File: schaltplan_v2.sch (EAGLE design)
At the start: 43 parts, among them T1 2N3565, T2 2N3565, T3 2N3565, T4 2N3565, T5 2N3565, T6 2N3565, T7 2N3565, T8 2N3565, X1 SSW-102-02-S-S-RA, X2 SSW-102-02-S-S-RA, X3 SSW-103-02-S-S-RA, X4 SSW-109-02-S-S-RA, X5 SSW-103-02-S-S-RA, X6 SSW-103-02-S-S-RA, X7 SSW-103-02-S-S-RA

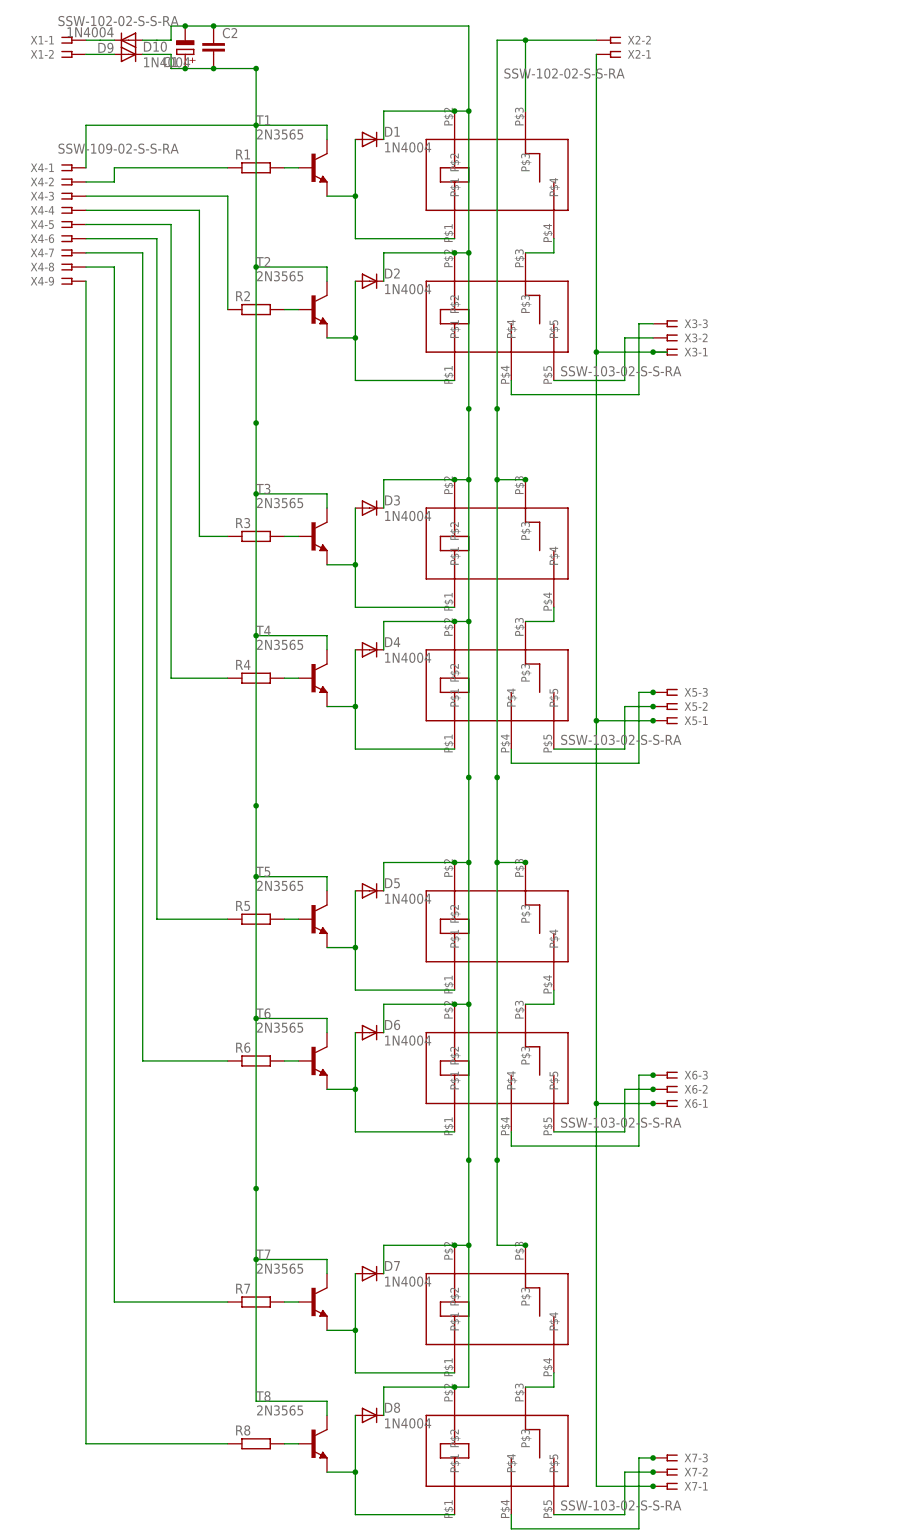
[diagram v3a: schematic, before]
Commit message: more fixes
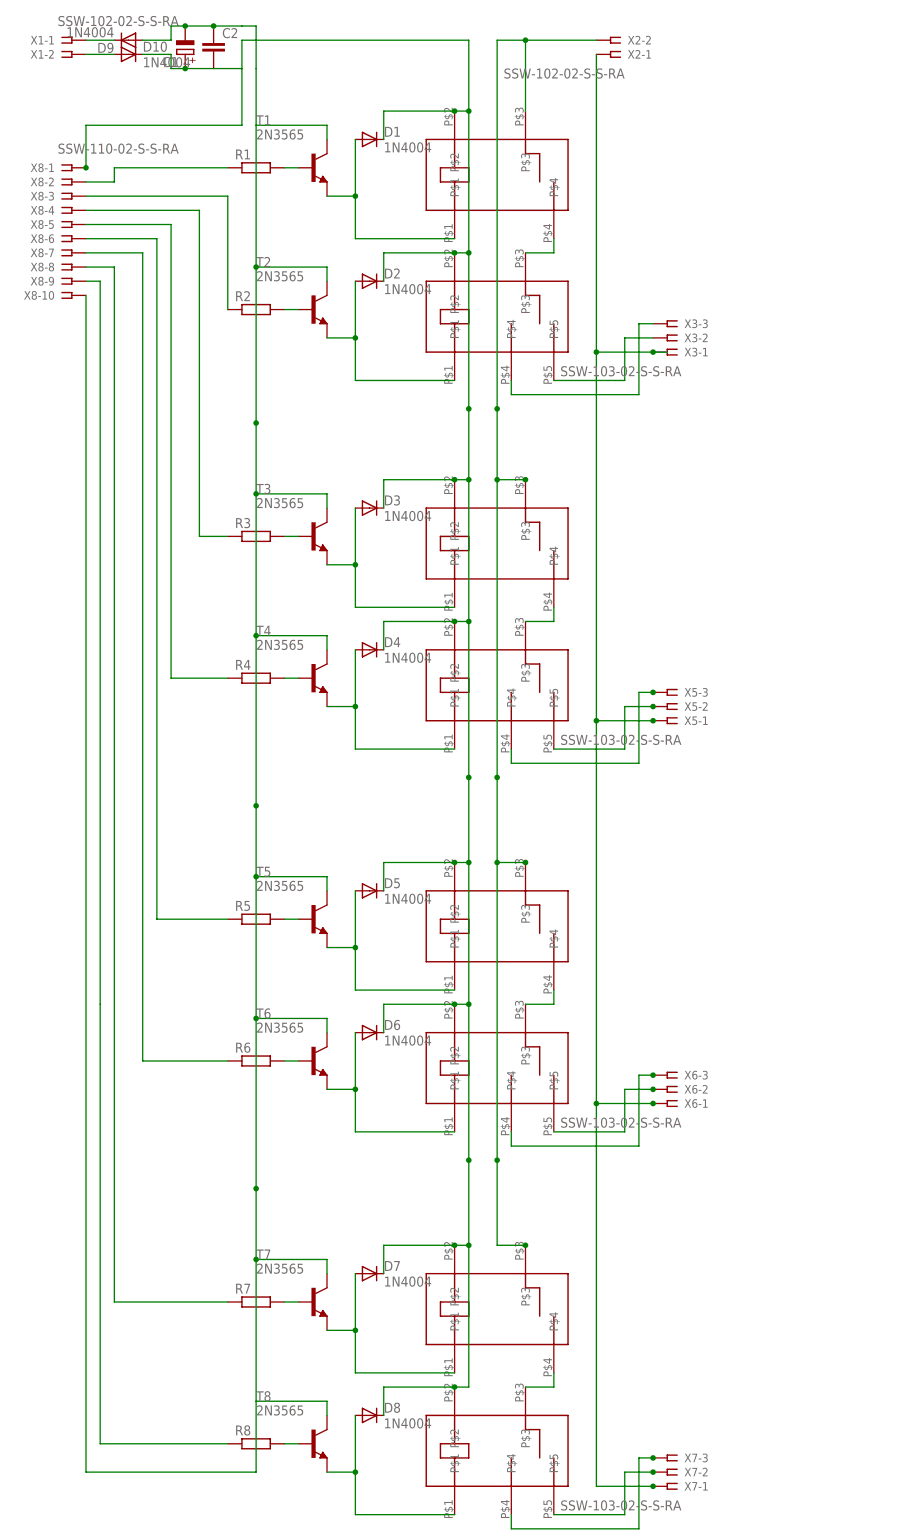
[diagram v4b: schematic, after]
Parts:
- removed X4: SSW-109-02-S-S-RA, con-samtec:SSW-109-02-S-S-RA
- added X8: SSW-110-02-S-S-RA, con-samtec:SSW-110-02-S-S-RA
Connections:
- removed net N$29 (its old number): C1.-, C2.1, D1.C, D2.C, D3.C, D4.C, D5.C, D6.C, D7.C, D8.C, D9.A, U$1.P$2, U$2.P$2, U$3.P$2, U$4.P$2, U$5.P$2, U$6.P$2, U$7.P$2, U$8.P$2
- new net N$19: C1.-, C2.1, D9.A, T1.C, T2.C, T3.C, T4.C, T5.C, T6.C, T7.C, T8.C, X8-10.1
- net N$11: now also X8-3.1; no longer X4-3.1
- net N$14: now also X8-4.1; no longer X4-4.1
- net N$23: now also X8-5.1; no longer X4-5.1
- net N$24: now also D1.C, D2.C, D3.C, D4.C, D5.C, D6.C, D7.C, D8.C, U$1.P$2, U$2.P$2, U$3.P$2, U$4.P$2, U$5.P$2, U$6.P$2, U$7.P$2, U$8.P$2, X8-1.1; no longer T1.C, T2.C, T3.C, T4.C, T5.C, T6.C, T7.C, T8.C, X4-1.1
- net N$26: now also X8-6.1; no longer X4-6.1
- net N$37: now also X8-7.1; no longer X4-7.1
- net N$49: now also X8-8.1; no longer X4-8.1
- net N$7: now also X8-9.1; no longer X4-9.1
- net N$9: now also X8-2.1; no longer X4-2.1
